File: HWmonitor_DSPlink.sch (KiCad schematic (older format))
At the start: 10 parts

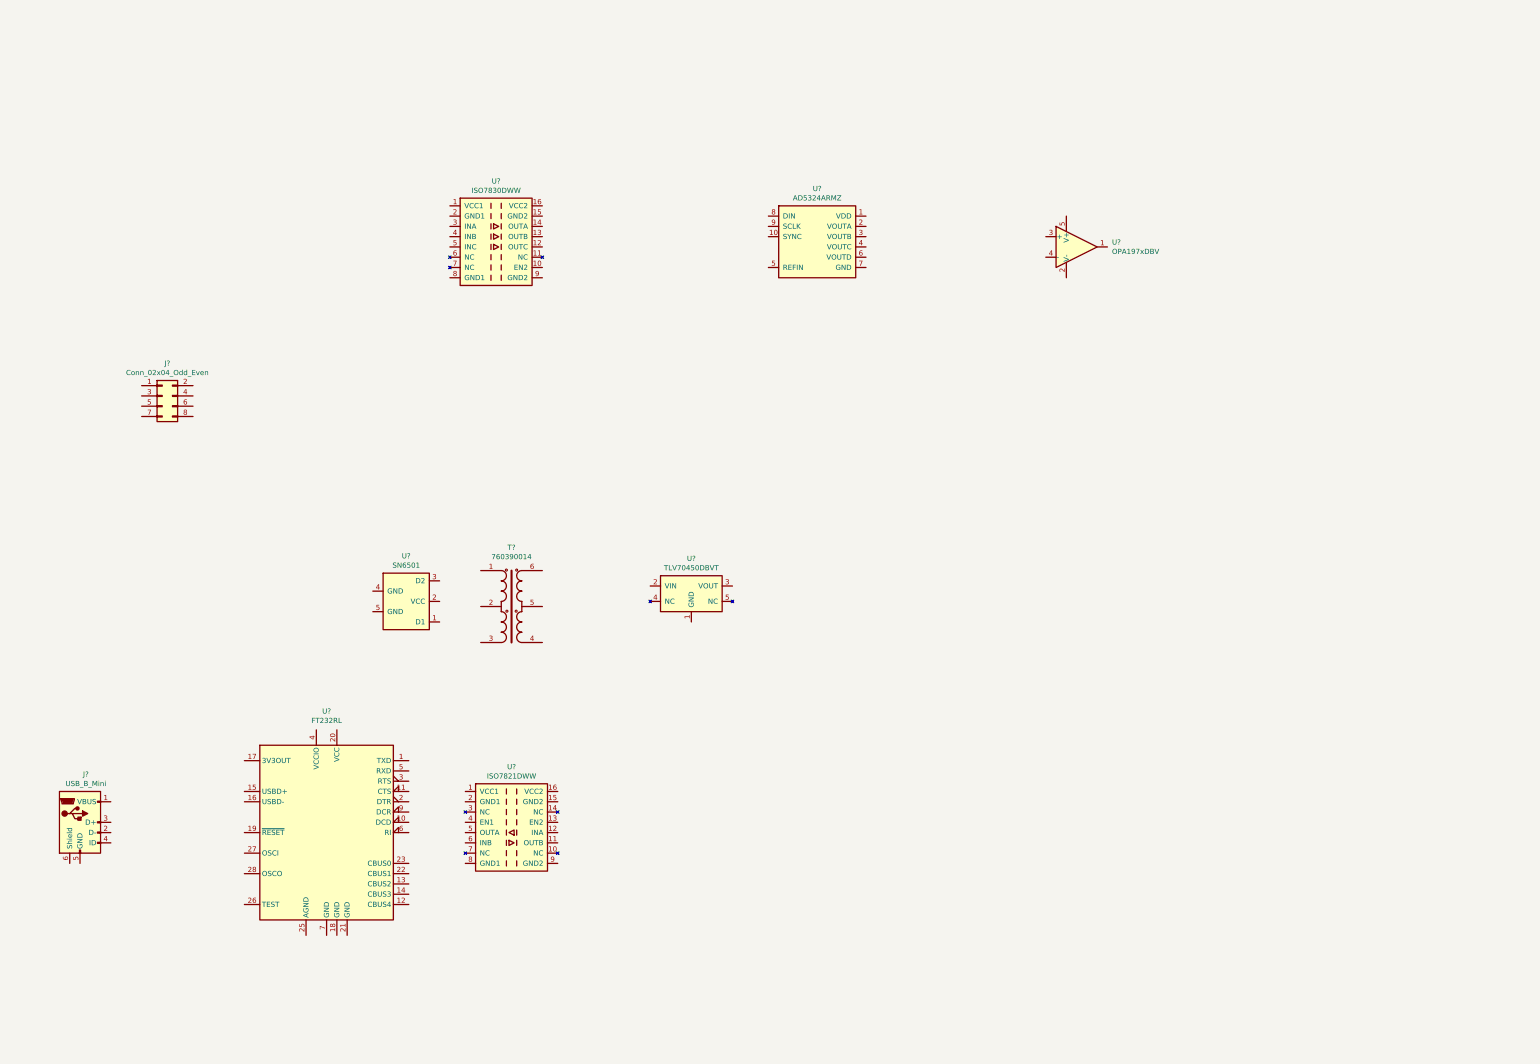
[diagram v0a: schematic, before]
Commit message: Schematic drawn!
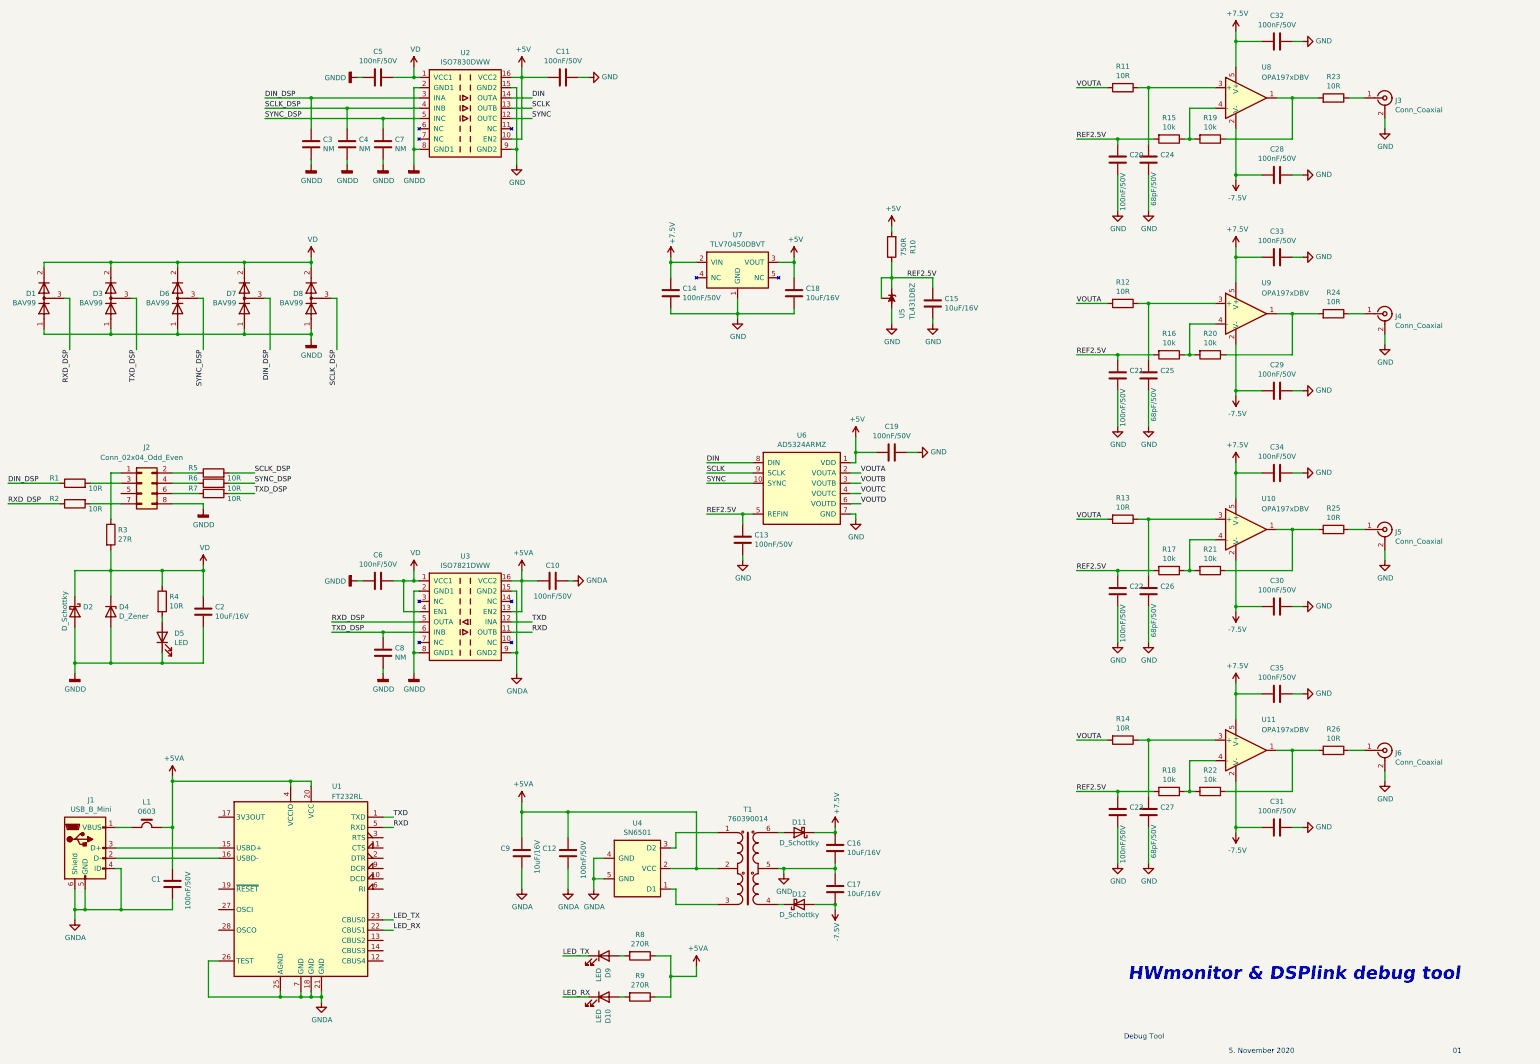
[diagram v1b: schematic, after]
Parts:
- removed J?: USB_B_Mini, symbol Connector:USB_B_Mini
- removed U?: FT232RL, Package_SO:SSOP-28_5.3x10.2mm_P0.65mm, symbol Interface_USB:FT232RL
- added C1, C10, C11, C12, C13, C14, C19, C20, C21, C22, C23, C28, C29, C30, C31, C32, C33, C34, C35, C5, C6: 100nF/50V, symbol Device:C
- added C15, C16, C17, C18, C2, C9: 10uF/16V, symbol Device:C
- added C24, C25, C26, C27: 68pF/50V, symbol Device:C
- added C3, C4, C7, C8: NM, symbol Device:C
- added D1, D3, D6, D7, D8: BAV99, Package_TO_SOT_SMD:SOT-23, symbol Diode:BAV99
- added D10, D5, D9: LED, symbol Device:LED
- added D11, D12, D2: D_Schottky, symbol Device:D_Schottky
- added D4: D_Zener, symbol Device:D_Zener
- added J1: USB_B_Mini, symbol Connector:USB_B_Mini
- added J3, J4, J5, J6: Conn_Coaxial, symbol Connector:Conn_Coaxial
- added L1: 0603, symbol #MyLibrary:Ferrite_Bead
- added R1, R11, R12, R13, R14, R2, R23, R24, R25, R26, R4, R5, R6, R7: 10R, symbol Device:R
- added R10: 750R, symbol Device:R
- added R15, R16, R17, R18, R19, R20, R21, R22: 10k, symbol Device:R
- added R3: 27R, symbol Device:R
- added R8, R9: 270R, symbol Device:R
- added U1: FT232RL, Package_SO:SSOP-28_5.3x10.2mm_P0.65mm, symbol Interface_USB:FT232RL
- added U10, U11, U9: OPA197xDBV, Package_TO_SOT_SMD:SOT-23-5, symbol Amplifier_Operational:OPA197xDBV
- added U5: TL431DBZ, Package_TO_SOT_SMD:SOT-23, symbol Reference_Voltage:TL431DBZ
- gave numbers to parts that had none: 8
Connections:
- net at T1.1: now also U4.3 (D2)
- net +5VA: now reaches T1.2
- net +5VA: now also U3.13 (EN2), U3.16 (VCC2), U4.2 (VCC), C1.1, C10.1, C12.1, C9.2, L1.2, R8.1, R9.1, U1.20 (VCC), U1.4 (VCCIO)
- net at T1.3: now also U4.1 (D1)
- net at T1.4: now also D12.1 (K)
- net GND: now reaches T1.5
- net GND: now also U2.15 (GND2), U2.9 (GND2), U6.7 (GND), U7.1 (GND), C11.2, C13.1, C14.1, C15.1, C16.1, C17.2, C18.1, C19.2, C20.1, C21.1, C22.1, C23.1, C24.1, C25.1, C26.1, C27.1, C28.1, C29.1, C30.1, C31.1, C32.1, C33.1, C34.1, C35.1, J3.2 (Ext), J4.2 (Ext), J5.2 (Ext), J6.2 (Ext), U5.3 (A)
- net at T1.6: now also D11.2 (A)
- net GNDA: now reaches U4.4 (GND)
- net GNDA: now also U3.15 (GND2), U3.9 (GND2), U4.5 (GND), C1.2, C10.2, C12.2, C9.1, J1.4 (ID), J1.5 (GND), J1.6 (Shield), U1.18 (GND), U1.21 (GND), U1.25 (AGND), U1.26 (TEST), U1.7 (GND)
- net at J2.1 (Pin_1): now also R3.1
- net at J2.2 (Pin_2): now also R5.1
- net at J2.3 (Pin_3): now also R1.2
- net at J2.4 (Pin_4): now also R6.1
- net at J2.6 (Pin_6): now also R7.1
- net at J2.7 (Pin_7): now also R2.2
- net GNDD: now reaches J2.8 (Pin_8)
- net GNDD: now also U2.2 (GND1), U2.8 (GND1), U3.2 (GND1), U3.8 (GND1), C2.1, C3.1, C4.1, C5.1, C6.1, C7.1, C8.1, D1.1 (K), D2.2 (A), D3.1 (K), D4.2 (A), D5.1 (K), D6.1 (K), D7.1 (K), D8.1 (K)
- net at U8.1: now also R19.1, R23.2
- net -7.5V: now reaches U8.2 (V-)
- net -7.5V: now also C17.1, C28.2, C29.2, C30.2, C31.2, D12.2 (A), U10.2 (V-), U11.2 (V-), U9.2 (V-)
- net at U8.3 (+): now also C24.2, R11.1
- net at U8.4 (-): now also R15.1, R19.2
- net +7.5V: now reaches U8.5 (V+)
- net +7.5V: now also U7.2 (VIN), C14.2, C16.2, C32.2, C33.2, C34.2, C35.2, D11.1 (K), U10.5 (V+), U11.5 (V+), U9.5 (V+)
- net VD: now reaches U3.1 (VCC1)
- net VD: now also U2.1 (VCC1), U3.4 (EN1), C2.2, C5.2, C6.2, D1.2 (A), D2.1 (K), D3.2 (A), D4.1 (K), D6.2 (A), D7.2 (A), D8.2 (A), R3.2, R4.1
- net RXD: now reaches U3.11 (OUTB)
- net RXD: now also U1.5 (RXD)
- net TXD: now reaches U3.12 (INA)
- net TXD: now also U1.1 (TXD)
- net RXD_DSP: now reaches U3.5 (OUTA)
- net RXD_DSP: now also D1.3 (K), R2.1
- net TXD_DSP: now reaches U3.6 (INB)
- net TXD_DSP: now also C8.2, D3.3 (K), R7.2
- net +5V: now reaches U2.10 (EN2)
- net +5V: now also U2.16 (VCC2), U6.1 (VDD), U7.3 (VOUT), C11.1, C18.2, C19.1, R10.2
- net SYNC: now reaches U2.12 (OUTC)
- net SYNC: now also U6.10 (SYNC)
- net SCLK: now reaches U2.13 (OUTB)
- net SCLK: now also U6.9 (SCLK)
- net DIN: now reaches U2.14 (OUTA)
- net DIN: now also U6.8 (DIN)
- net DIN_DSP: now reaches U2.3 (INA)
- net DIN_DSP: now also C3.2, D7.3 (K), R1.1
- net SCLK_DSP: now reaches U2.4 (INB)
- net SCLK_DSP: now also C4.2, D8.3 (K), R5.2
- net SYNC_DSP: now reaches U2.5 (INC)
- net SYNC_DSP: now also C7.2, D6.3 (K), R6.2
- net VOUTA: now reaches U6.2 (VOUTA)
- net VOUTA: now also R11.2, R12.2, R13.2, R14.2
- net VOUTB: now reaches U6.3 (VOUTB)
- net VOUTC: now reaches U6.4 (VOUTC)
- net REF2.5V: now reaches U6.5 (REFIN)
- net REF2.5V: now also C13.2, C15.2, C20.2, C21.2, C22.2, C23.2, R10.1, R15.2, R16.2, R17.2, R18.2, U5.1 (K), U5.2 (REF)
- net VOUTD: now reaches U6.6 (VOUTD)
- new net: J3.1 (In), R23.1
- new net: D5.2 (A), R4.2
- new net: J1.3 (D+), U1.15 (USBD+)
- new net: J1.2 (D-), U1.16 (USBD-)
- new net: J1.1 (VBUS), L1.1
- new net: D9.2 (A), R8.2
- new net: D10.2 (A), R9.2
- new net: R20.1, R24.2, U9.1
- new net: C25.2, R12.1, U9.3 (+)
- new net: R16.1, R20.2, U9.4 (-)
- new net: J4.1 (In), R24.1
- new net: R21.1, R25.2, U10.1
- new net: C26.2, R13.1, U10.3 (+)
- new net: R17.1, R21.2, U10.4 (-)
- new net: J5.1 (In), R25.1
- new net: R22.1, R26.2, U11.1
- new net: C27.2, R14.1, U11.3 (+)
- new net: R18.1, R22.2, U11.4 (-)
- new net: J6.1 (In), R26.1
- new net LED_RX: D10.1 (K), U1.22 (CBUS1)
- new net LED_TX: D9.1 (K), U1.23 (CBUS0)
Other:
- note added: "01"
- note added: "5. November 2020"
- note added: "Debug Tool"
- note added: "HWmonitor & DSPlink debug tool"
- moved on the sheet: J2, T1, U2, U3, U4, U6, U7, U8
